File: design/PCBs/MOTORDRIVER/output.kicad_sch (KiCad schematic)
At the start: 8 parts, among them J2 1-84952-1, J3 1-84952-1, J4 1-84952-1

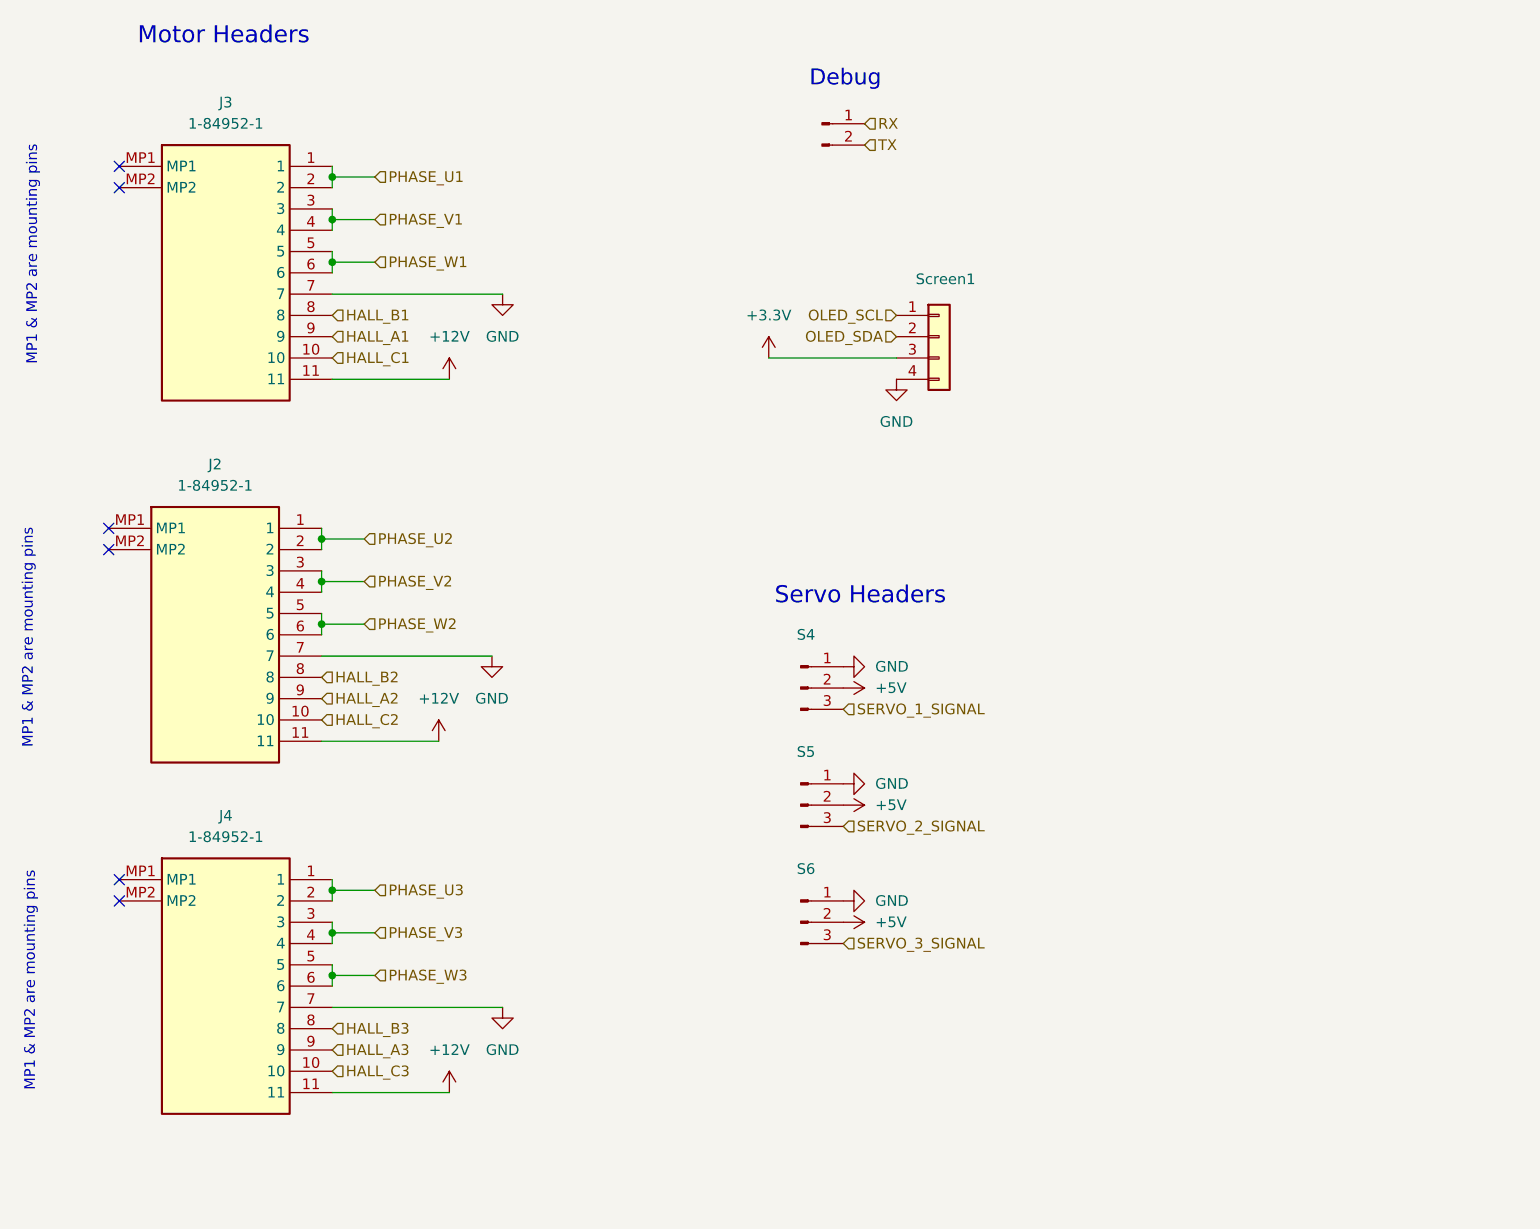
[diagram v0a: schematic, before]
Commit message: finished 12v voltage, The components for alost all ICs need values. Cleaned up a bit
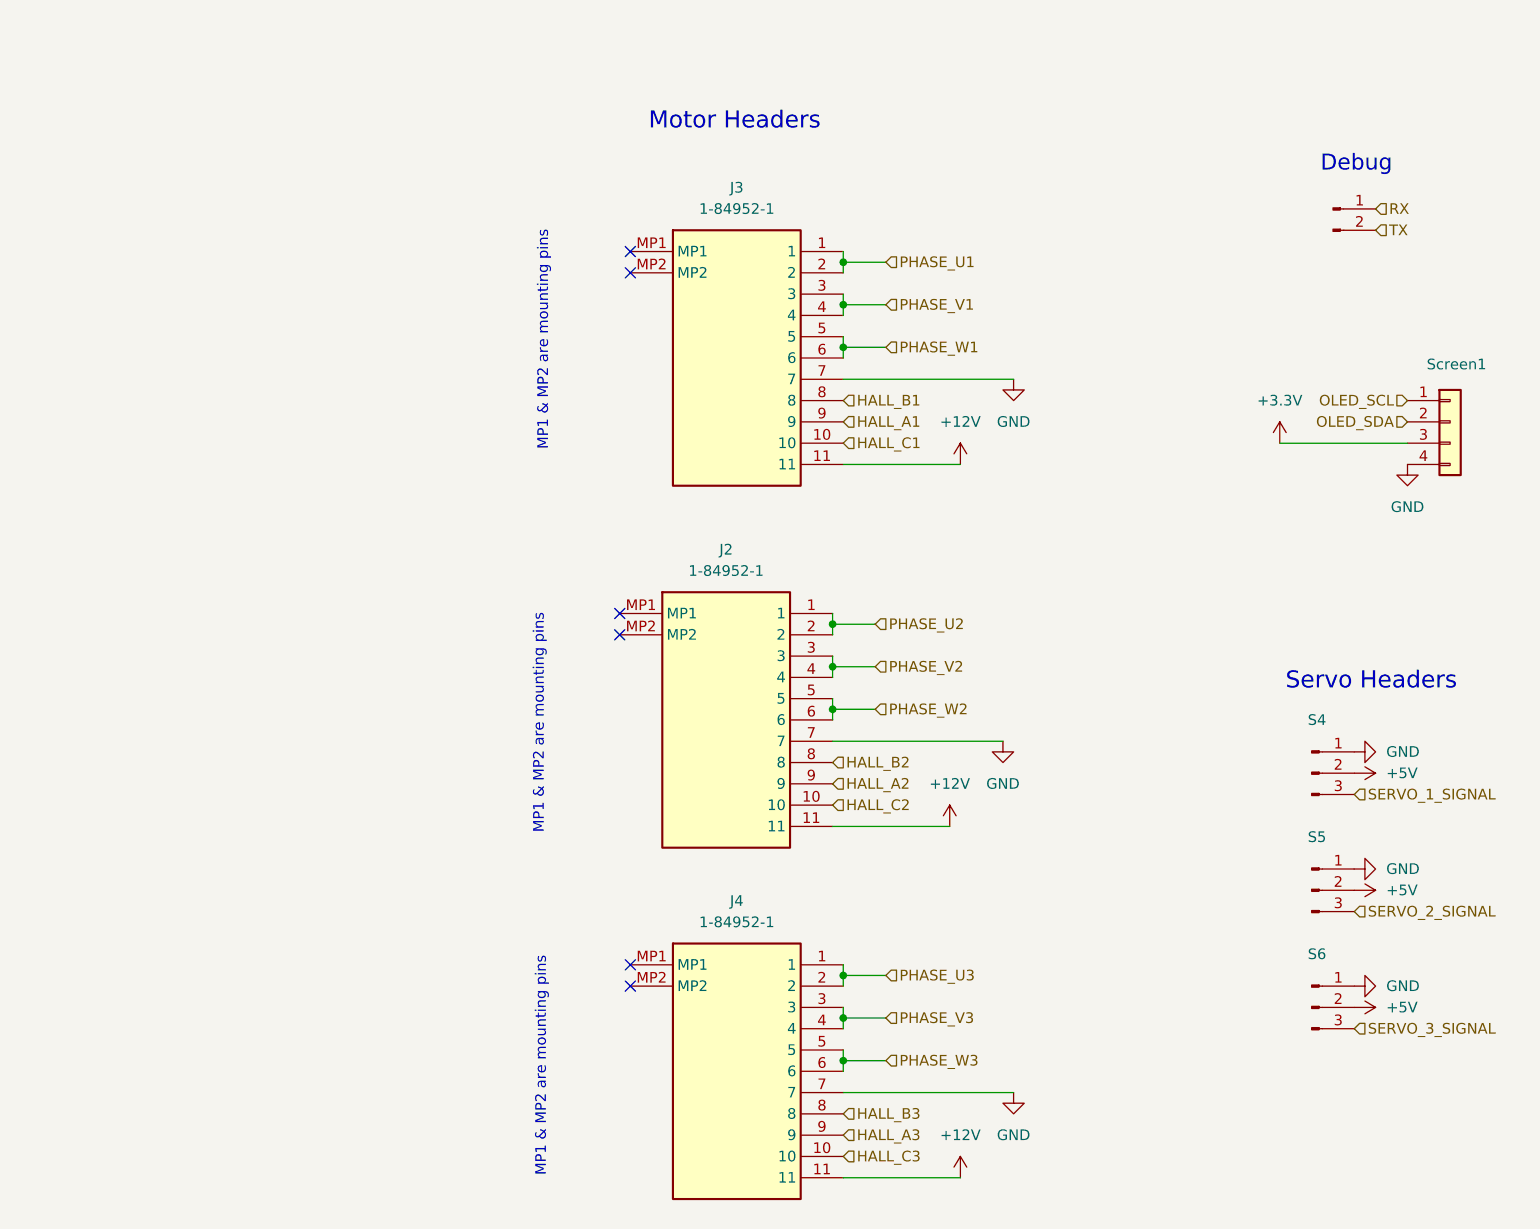
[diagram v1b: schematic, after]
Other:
- moved on the sheet: J2, J3, J4, S4, S5, S6, Screen1
